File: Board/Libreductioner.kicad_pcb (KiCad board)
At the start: 2 copper layers, 50.2 x 73 mm, 46 parts, among them J1 Conn_01x02_Male, J2 Conn_01x02_Male, J3 Conn_01x02_Male, J4 Conn_01x02_Male, J5 Conn_01x02_Male, J6 Conn_01x02_Male, Q1 IRF3205, U1 ATMEGA168A-AU, U2 PC817, U3 PC817, U4 LM1117-5.0, Y1 Crystal

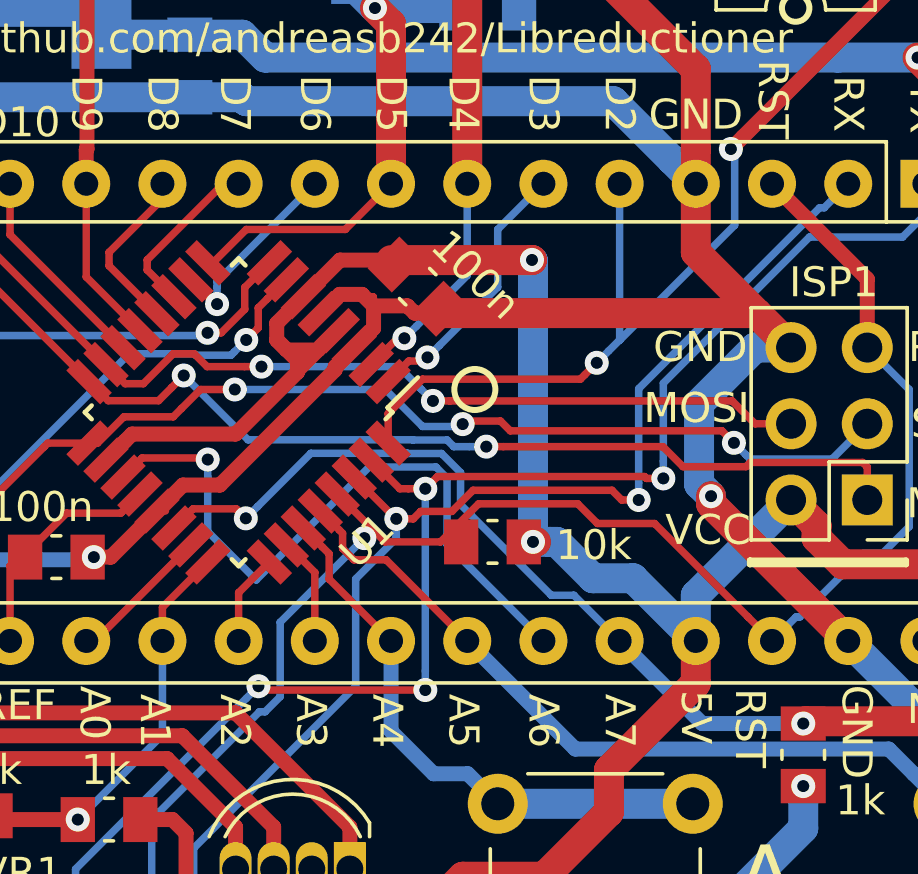
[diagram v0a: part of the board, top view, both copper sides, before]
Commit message: Added gerber files for production
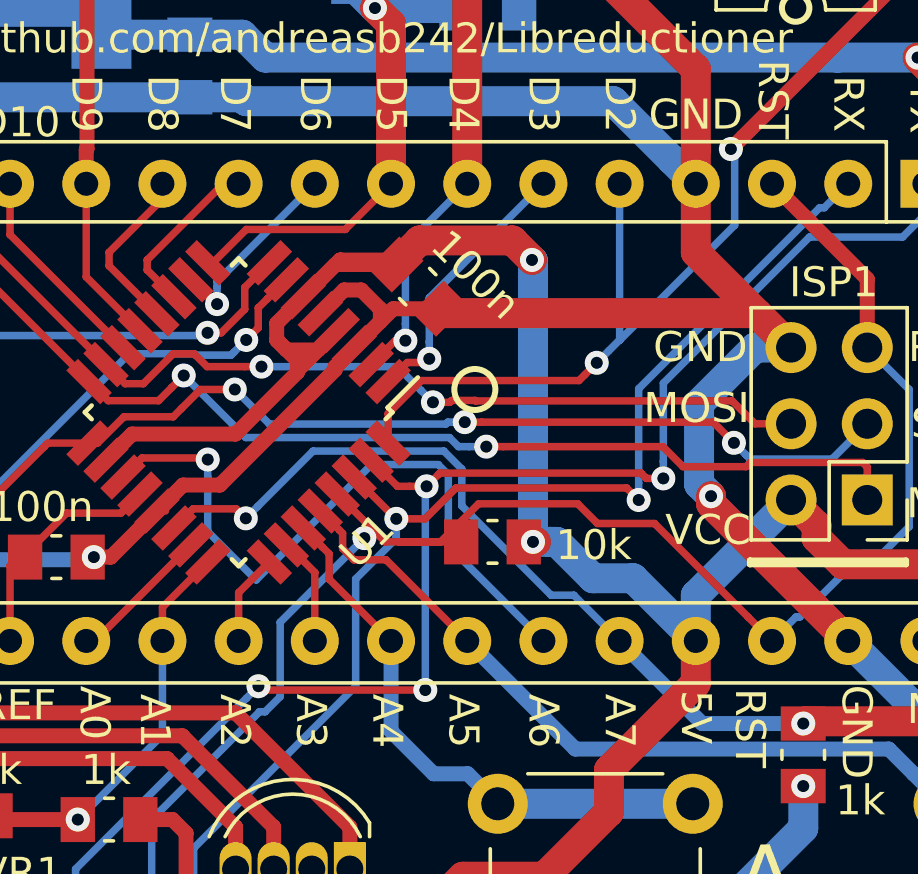
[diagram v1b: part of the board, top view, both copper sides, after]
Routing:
- net VCC: track 147.9 -> 151.9 mm
- net GND: track 482.3 -> 480.1 mm
- net /RESET: track 53.6 -> 55.6 mm
